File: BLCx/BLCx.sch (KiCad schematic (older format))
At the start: 20 parts

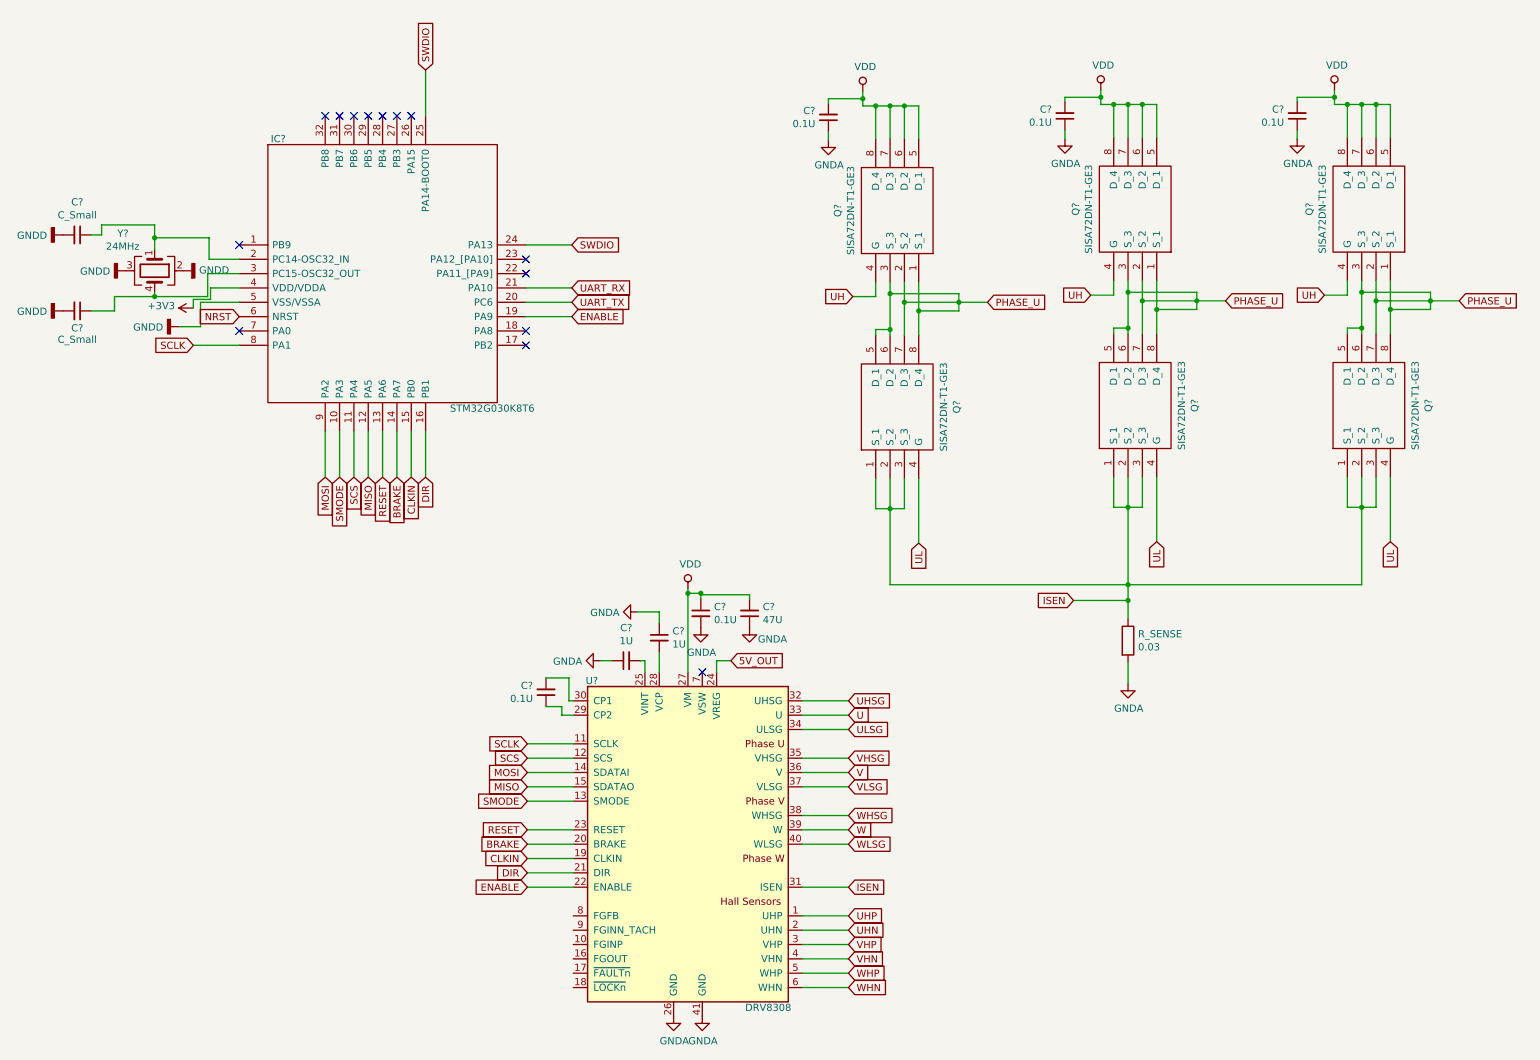
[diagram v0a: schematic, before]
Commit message: Add files via upload
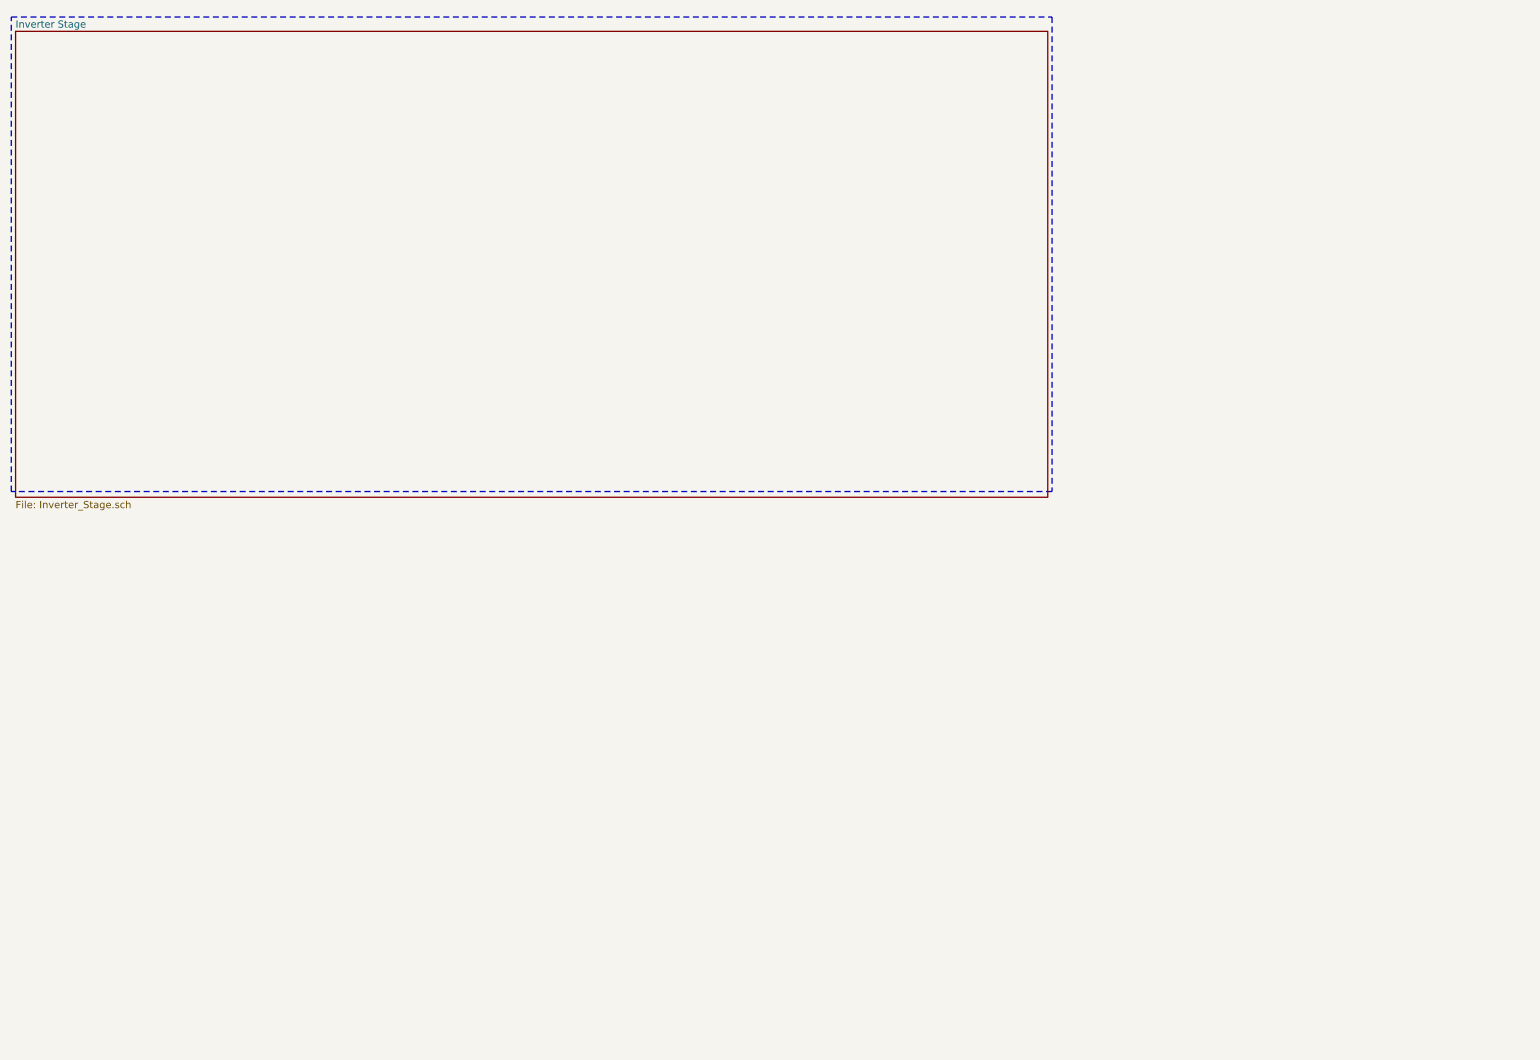
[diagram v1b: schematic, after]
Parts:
- removed C? (x5): 0.1U, symbol Device:C_Small
- removed C? (x2): 1U, symbol Device:C_Small
- removed C?: 47U, symbol Device:C_Small
- removed C? (x2): C_Small, symbol Device:C_Small
- removed IC?: STM32G030K8T6, ASSETS:QFP80P900X900X160-32N, symbol Regular_Use:STM32G030K8T6
- removed Q? (x6): SISA72DN-T1-GE3, ASSETS:SiSA72DN, symbol Regular_Use:SISA72DN-T1-GE3
- removed R_SENSE: 0.03, symbol Device:R
- removed U?: DRV8308, Package_DFN_QFN:Texas_S-PVQFN-N40_EP3.52x2.62mm, symbol Driver_Motor:DRV8308
- removed Y?: 24MHz, symbol Device:Crystal_GND23
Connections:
- no-connect marks 14 -> 0
